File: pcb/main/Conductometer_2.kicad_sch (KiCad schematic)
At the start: 30 parts

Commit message: fix: symbol libraries in Kicad 6.0
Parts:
- C10, C32, C4: value (none) -> 10u; footprint (none) -> Capacitor_SMD:C_0805_2012Metric_Pad1.18x1.45mm_HandSolder; symbol pHMeter-rescue:CP1-Device -> Device:C_Polarized
- C12, C2, C34, C8: value (none) -> 100n; footprint (none) -> Capacitor_SMD:C_0805_2012Metric_Pad1.18x1.45mm_HandSolder; symbol pHMeter-rescue:C-Device -> Device:C
- C30: symbol pHMeter-rescue:CP1-Device -> Device:C_Polarized
- C35: value (none) -> 20p; footprint (none) -> Capacitor_SMD:C_0805_2012Metric_Pad1.18x1.45mm_HandSolder; symbol pHMeter-rescue:C-Device -> Device:C
- C36, C37: value (none) -> 100u; footprint (none) -> Capacitor_SMD:CP_Elec_8x10; symbol pHMeter-rescue:CP1-Device -> Device:C_Polarized
- C5: value (none) -> 1.5n; footprint (none) -> Capacitor_SMD:C_0805_2012Metric_Pad1.18x1.45mm_HandSolder; symbol pHMeter-rescue:C-Device -> Device:C
- D1: symbol pHMeter-rescue:1N4148W-Diode -> Diode:1N4148W
- D2: value (none) -> 1N4148W; footprint (none) -> Diode_SMD:D_SOD-123; symbol pHMeter-rescue:1N4148W-Diode -> Diode:1N4148W
- D6: symbol pHMeter-rescue:1N5819-Diode -> Diode:1N5819
- J2: symbol pHMeter-rescue:Conn_Coaxial_Power-Connector -> Connector:Conn_Coaxial_Power
- R1: value (none) -> 820; footprint (none) -> Resistor_SMD:R_0805_2012Metric_Pad1.20x1.40mm_HandSolder; symbol pHMeter-rescue:R-Device -> Device:R
- R10, R12, R5, R7, R8, R9: value (none) -> 36k; footprint (none) -> Resistor_SMD:R_0805_2012Metric_Pad1.20x1.40mm_HandSolder; symbol pHMeter-rescue:R-Device -> Device:R
- R17: value (none) -> 51k; footprint (none) -> Resistor_SMD:R_0805_2012Metric_Pad1.20x1.40mm_HandSolder; symbol pHMeter-rescue:R-Device -> Device:R
- R18: value (none) -> 2k; footprint (none) -> Resistor_SMD:R_0805_2012Metric_Pad1.20x1.40mm_HandSolder; symbol pHMeter-rescue:R-Device -> Device:R
- R2: value (none) -> 100k; footprint (none) -> Resistor_SMD:R_0805_2012Metric_Pad1.20x1.40mm_HandSolder; symbol pHMeter-rescue:R-Device -> Device:R
- R6: value (none) -> 10k; footprint (none) -> Resistor_SMD:R_0805_2012Metric_Pad1.20x1.40mm_HandSolder; symbol pHMeter-rescue:R-Device -> Device:R
- U10: value (none) -> LM2660M; footprint (none) -> pHMeter:LM2660M
- U2: value (none) -> TLV6004PW; footprint (none) -> Package_SO:TSSOP-14_4.4x5mm_P0.65mm
- U8: value (none) -> CD4060BM; footprint (none) -> pHMeter:CD4060BM
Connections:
- net Vin is gone; now on net +3V3: U2.4 (V+)
- net CT1: now also J2.1 (In), R18.2
- net CT2: now also J2.2 (Ext), R1.2
- net GND: now also C10.2, C12.2, C2.2, C30.2, C32.1, C34.2, C35.2, C37.1, C4.1, C8.2, D6.2 (A)
- net Vout: now also C35.1, D6.1 (K), R12.1
- net at U2.2 (-): now also R17.1, R18.1
- net at U2.7: now also R1.1, R5.2
- net at U2.8: now also D1.1 (K), D2.2 (A)
- net at U2.9 (-): now also R5.1, R7.2, R8.2
- net -3V3: now reaches U2.11 (V-)
- net -3V3: now also C2.1, C32.2, C34.1, C37.2, C4.2, U10.5 (OUT), U8.12 (RESET), U8.8 (VSS)
- net at U8.10 (O): now also R6.1
- net at U8.11 (I): now also R2.1
- net +3V3: now reaches U8.16 (VDD)
- net +3V3: now also C10.1, C12.1, C30.1, C8.1, U10.8 (V+)
- net at U8.7 (Q4): now also R17.2
- net at U8.9 (O): now also C5.1
- net at U10.2 (CAP+): now also C36.1
- net at U10.4 (CAP-): now also C36.2
- net at U2.12 (+): now also R10.2, R9.1
- net at U2.13 (-): now also D2.1 (K), R8.1
- net at U2.14: now also R10.1, R12.2
- new net: C5.2, R2.2, R6.2
- new net: D1.2 (A), R7.1, R9.2

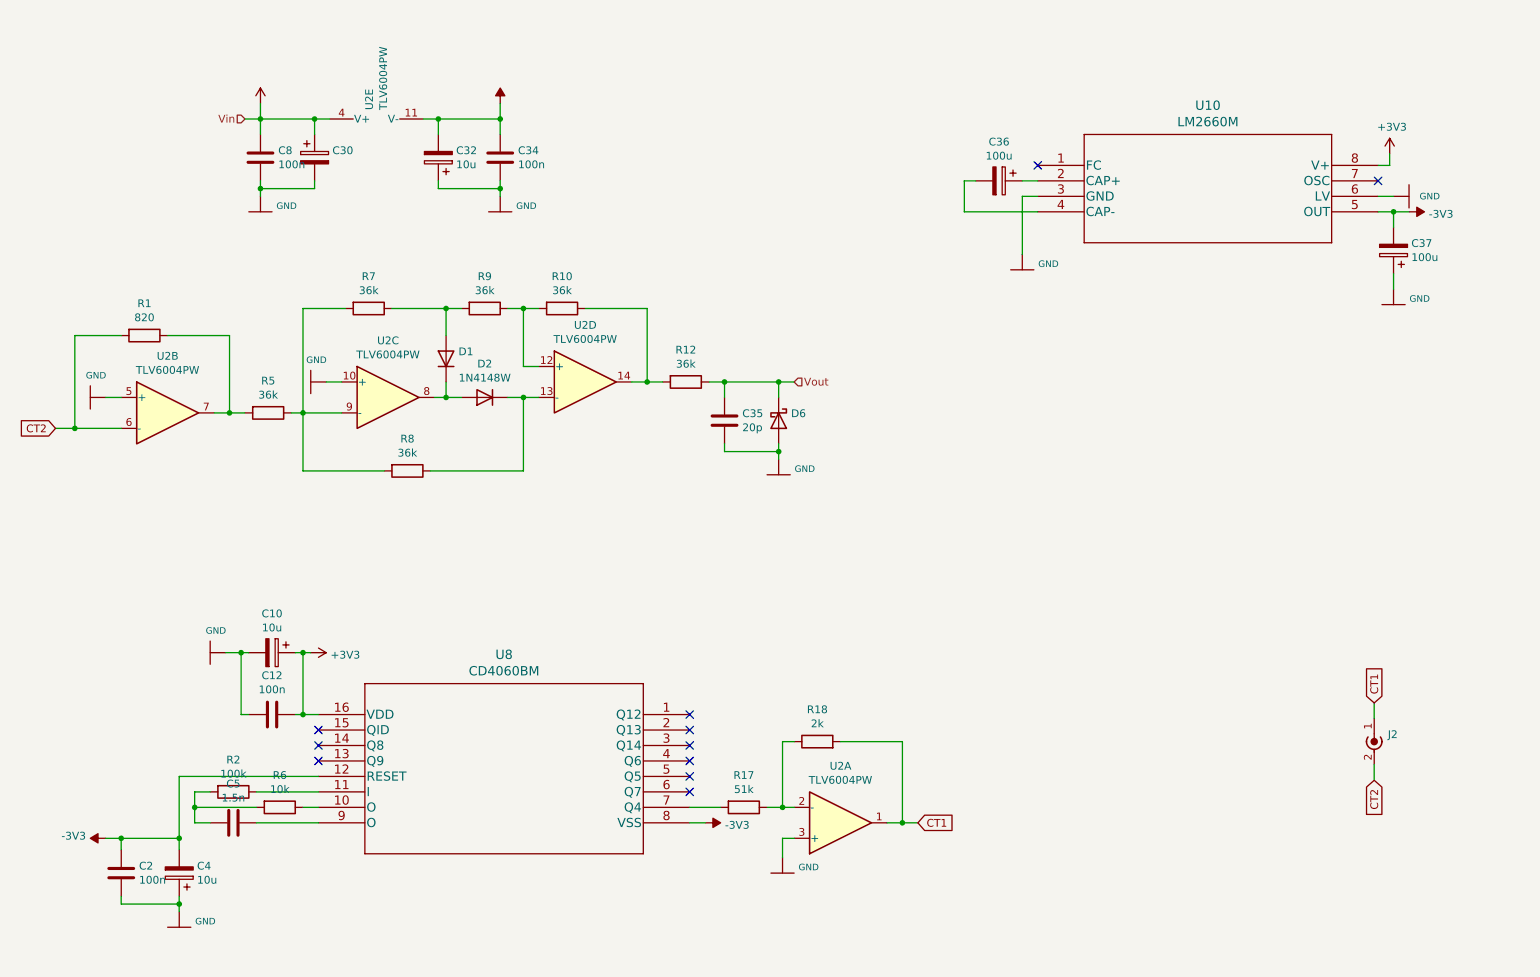
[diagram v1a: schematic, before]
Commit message: fix: 3D model libraries in Kicad 6.0
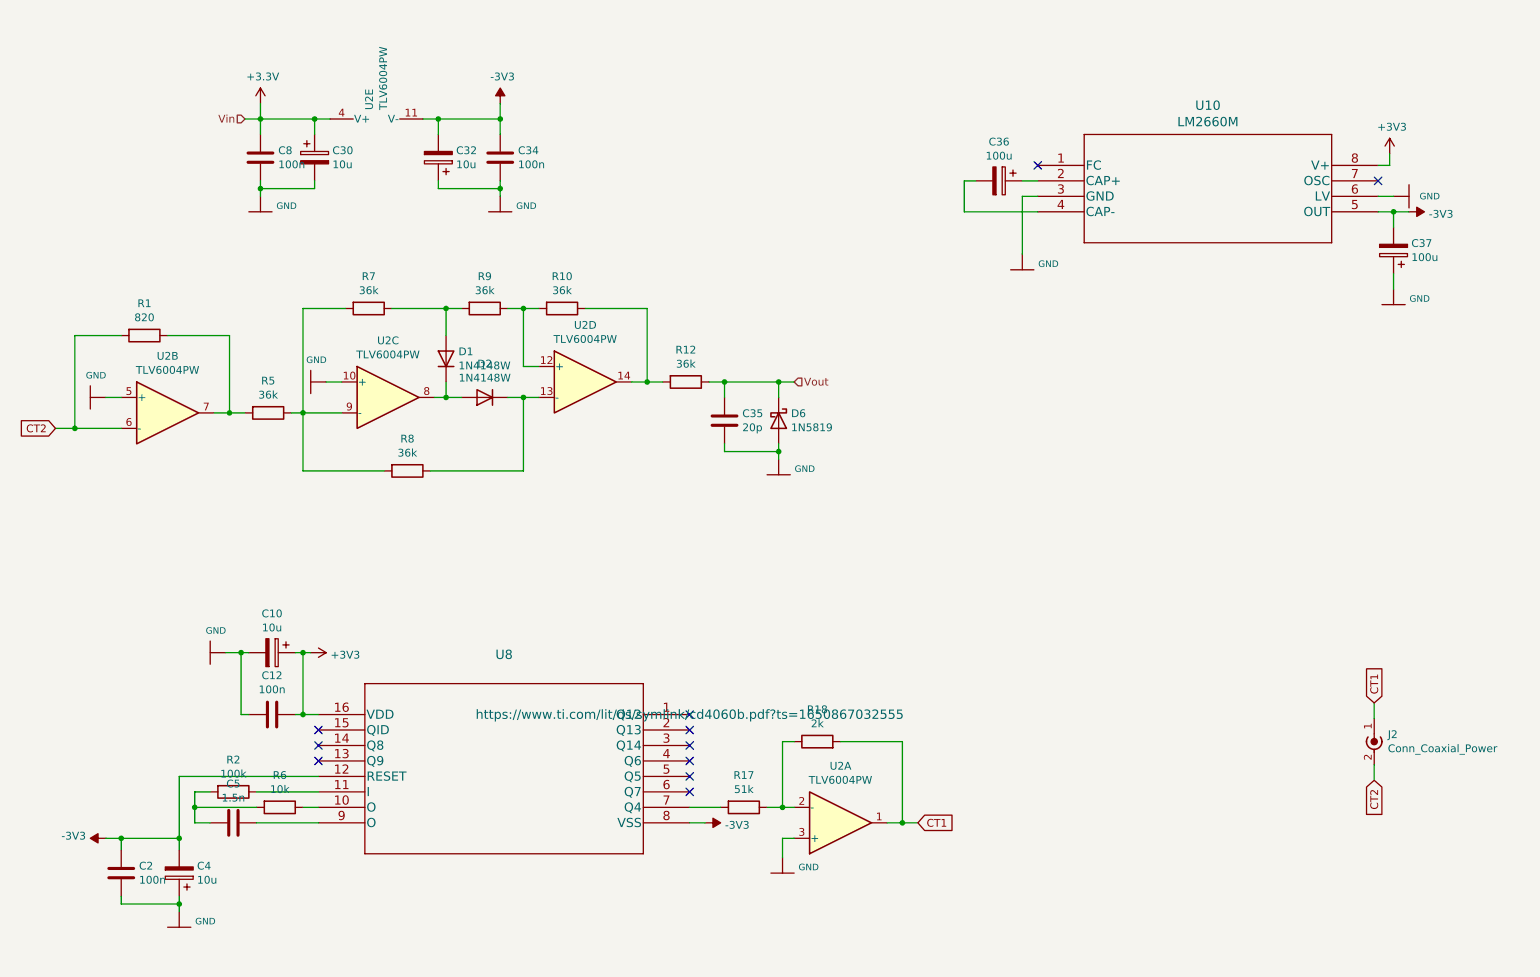
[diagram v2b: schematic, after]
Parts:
- C30: value (none) -> 10u; footprint (none) -> Capacitor_SMD:C_0805_2012Metric_Pad1.18x1.45mm_HandSolder
- D1: value (none) -> 1N4148W; footprint (none) -> Diode_SMD:D_SOD-123
- D6: value (none) -> 1N5819; footprint (none) -> Diode_SMD:D_SOD-123
- J2: value (none) -> Conn_Coaxial_Power; footprint (none) -> Connector_Coaxial:BNC_TEConnectivity_1478204_Vertical
- U8: value CD4060BM -> (none); footprint pHMeter:CD4060BM -> (none)
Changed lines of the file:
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@@
       (effects (font (size 1.524 1.524)))
     )
-    (property "Value" "CD4060BM" (id 1) (at 107.315 115.4176 0)
+    (property "Value" "" (id 1) (at 107.315 115.4176 0)
       (effects (font (size 1.524 1.524)))
     )
-    (property "Footprint" "pHMeter:CD4060BM" (id 2) (at 107.315 116.459 0)
+    (property "Footprint" "" (id 2) (at 107.315 116.459 0)
       (effects (font (size 1.524 1.524)) hide)
     )
-    (property "Datasheet" "" (id 3) (at 137.795 122.555 0)
+    (property "Datasheet" "https://www.ti.com/lit/ds/symlink/cd4060b.pdf?ts=1650867032555" (id 3) (at 137.795 122.555 0)
       (effects (font (size 1.524 1.524)))
     )
@@
       (effects (font (size 1.27 1.27)) (justify left))
     )
-    (property "Value" "" (id 1) (at 79.121 32.258 0)
-      (effects (font (size 1.27 1.27)) (justify left))
-    )
-    (property "Footprint" "" (id 2) (at 76.2 31.115 0)
+    (property "Value" "10u" (id 1) (at 79.121 32.258 0)
+      (effects (font (size 1.27 1.27)) (justify left))
+    )
+    (property "Footprint" "Capacitor_SMD:C_0805_2012Metric_Pad1.18x1.45mm_HandSolder" (id 2) (at 76.2 31.115 0)
       (effects (font (size 1.27 1.27)) hide)
     )
@@
       (effects (font (size 1.27 1.27)) hide)
     )
-    (property "Value" "" (id 1) (at 67.691 17.8308 0))
+    (property "Value" "+3.3V" (id 1) (at 67.691 17.8308 0))
     (property "Footprint" "" (id 2) (at 67.31 22.225 0)
       (effects (font (size 1.27 1.27)) hide)
@@
       (effects (font (size 1.27 1.27)) hide)
     )
-    (property "Value" "" (id 1) (at 107.061 17.8308 0))
+    (property "Value" "-3V3" (id 1) (at 107.061 17.8308 0))
     (property "Footprint" "" (id 2) (at 106.68 22.225 0)
       (effects (font (size 1.27 1.27)) hide)
@@
       (effects (font (size 1.27 1.27)) (justify left))
     )
-    (property "Value" "" (id 1) (at 252.4252 128.143 0)
-      (effects (font (size 1.27 1.27)) (justify left))
-    )
-    (property "Footprint" "" (id 2) (at 250.19 127 0)
+    (property "Value" "Conn_Coaxial_Power" (id 1) (at 252.4252 128.143 0)
+      (effects (font (size 1.27 1.27)) (justify left))
+    )
+    (property "Footprint" "Connector_Coaxial:BNC_TEConnectivity_1478204_Vertical" (id 2) (at 250.19 127 0)
       (effects (font (size 1.27 1.27)) hide)
     )
@@
       (effects (font (size 1.27 1.27)) (justify right))
     )
-    (property "Value" "" (id 1) (at 99.822 65.278 90)
+    (property "Value" "1N4148W" (id 1) (at 99.822 65.278 90)
       (effects (font (size 1.27 1.27)) (justify right))
     )
-    (property "Footprint" "" (id 2) (at 102.235 64.135 0)
+    (property "Footprint" "Diode_SMD:D_SOD-123" (id 2) (at 102.235 64.135 0)
       (effects (font (size 1.27 1.27)) hide)
     )
@@
       (effects (font (size 1.27 1.27)) (justify left))
     )
-    (property "Value" "" (id 1) (at 154.432 75.438 90)
-      (effects (font (size 1.27 1.27)) (justify left))
-    )
-    (property "Footprint" "" (id 2) (at 147.955 74.295 0)
-      (effects (font (size 1.27 1.27)) hide)
-    )
+    (property "Value" "1N5819" (id 1) (at 154.432 75.438 90)
+      (effects (font (size 1.27 1.27)) (justify left))
+    )
+    (property "Footprint" "Diode_SMD:D_SOD-123" (id 2) (at 147.955 74.295 0)
+      (effects (font (size 1.27 1.27)) hide)
+    )

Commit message: fix: standard footprint for R and C, BOM updated
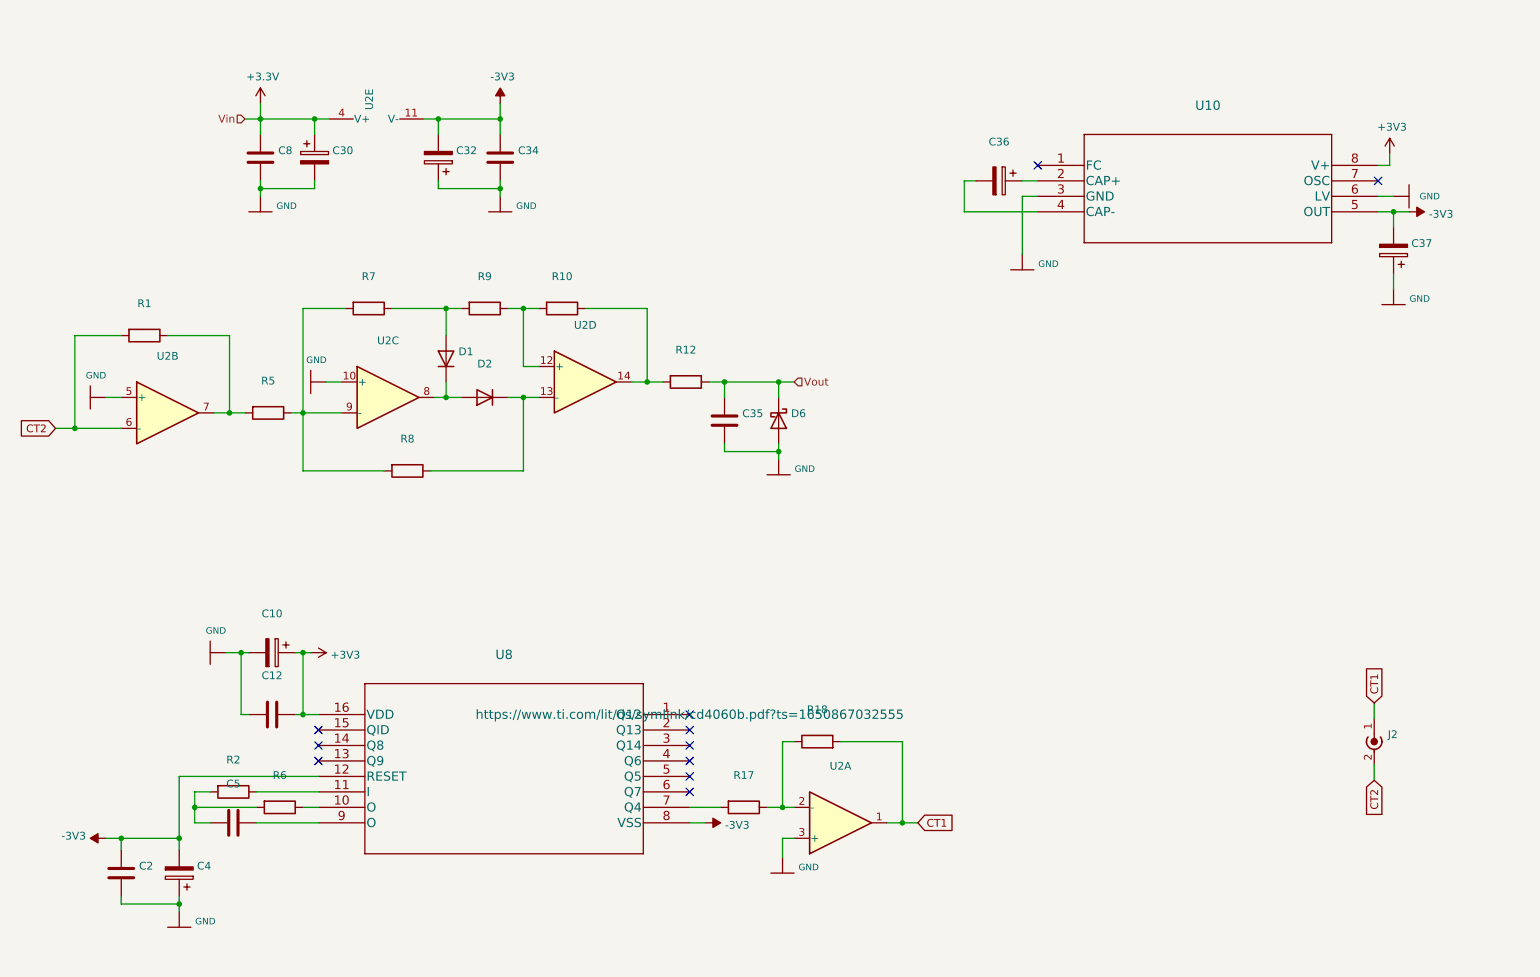
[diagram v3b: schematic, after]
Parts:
- C10, C30, C32, C4: value 10u -> (none); footprint Capacitor_SMD:C_0805_2012Metric_Pad1.18x1.45mm_HandSolder -> (none); MFN (none) -> Wurth Elektronik; MFP (none) -> 885012207072; S1PL (none) -> https://www.mouser.com/ProductDetail/Wurth-Elektronik/88501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; S1PN (none) -> 710-885012207072
- C12, C2, C34, C8: value 100n -> (none); footprint Capacitor_SMD:C_0805_2012Metric_Pad1.18x1.45mm_HandSolder -> (none); MFN (none) -> Wurth Elektronik; MFP (none) -> 885012207072; S1PL (none) -> https://www.mouser.com/ProductDetail/Wurth-Elektronik/88501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; S1PN (none) -> 710-885012207072
- C35: value 20p -> (none); footprint Capacitor_SMD:C_0805_2012Metric_Pad1.18x1.45mm_HandSolder -> (none); MFN (none) -> KEMET; MFP (none) -> C0805C200J5HACTU; S1PL (none) -> https://www.mouser.com/ProductDetail/KEMET/C0805C200J5HACTU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; S1PN (none) -> 80-C0805C200J5HACTU
- C36, C37: value 100u -> (none); footprint Capacitor_SMD:CP_Elec_8x10 -> (none); MFN (none) -> Cornell Dubilier - CDE; MFP (none) -> AVE107M35F24T-F; S1PL (none) -> https://www.mouser.com/ProductDetail/Cornell-Dubilier-CDE/A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; S1PN (none) -> 598-AVE107M35F24T-F
- C5: value 1.5n -> (none); footprint Capacitor_SMD:C_0805_2012Metric_Pad1.18x1.45mm_HandSolder -> (none); MFN (none) -> Wurth Elektronik; MFP (none) -> 885012207087; S1PL (none) -> https://www.mouser.com/ProductDetail/Wurth-Elektronik/88501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; S1PN (none) -> 710-885012207087
- D1, D2: value 1N4148W -> (none); footprint Diode_SMD:D_SOD-123 -> (none)
- D6: value 1N5819 -> (none); footprint Diode_SMD:D_SOD-123 -> (none)
- J2: value Conn_Coaxial_Power -> (none); footprint Connector_Coaxial:BNC_TEConnectivity_1478204_Vertical -> (none)
- R1: value 820 -> (none); footprint Resistor_SMD:R_0805_2012Metric_Pad1.20x1.40mm_HandSolder -> (none)
- R10, R12, R5, R7, R8, R9: value 36k -> (none); footprint Resistor_SMD:R_0805_2012Metric_Pad1.20x1.40mm_HandSolder -> (none)
- R17: value 51k -> (none); footprint Resistor_SMD:R_0805_2012Metric_Pad1.20x1.40mm_HandSolder -> (none)
- R18: value 2k -> (none); footprint Resistor_SMD:R_0805_2012Metric_Pad1.20x1.40mm_HandSolder -> (none)
- R2: value 100k -> (none); footprint Resistor_SMD:R_0805_2012Metric_Pad1.20x1.40mm_HandSolder -> (none)
- R6: value 10k -> (none); footprint Resistor_SMD:R_0805_2012Metric_Pad1.20x1.40mm_HandSolder -> (none)
- U10: value LM2660M -> (none); footprint pHMeter:LM2660M -> (none)
- U2: value TLV6004PW -> (none); footprint Package_SO:TSSOP-14_4.4x5mm_P0.65mm -> (none)
